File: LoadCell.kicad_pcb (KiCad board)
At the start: 2 copper layers, 51.1 x 18.5 mm, 62 parts, among them J1 M20-8760242, J2 0.100_1X4, J3 M20-8760242, J4 0.100_1X4, J5 M20-8760242, J6 0.100_1X4, J7 M20-8760242, J8 0.100_1X4, U1 L78L12ABUTR, U2 LM321SN3T1G, U3 L78L12ABUTR, U4 LM321SN3T1G, U5 L78L12ABUTR, U6 LM321SN3T1G, U7 L78L12ABUTR, U8 LM321SN3T1G

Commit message: Submitted to OSHpark
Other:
- rule pad_to_mask_clearance: 0.2 -> 0.0762
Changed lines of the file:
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@@
     (links 99)
     (no_connects 0)
-    (area 101.524999 82.982999 152.729001 101.675001)
+    (area 99.1 81.637 154.910797 105.713857)
     (thickness 1.6)
     (drawings 9)
@@
     (pad_size 1.45 1.45)
     (pad_drill 0.9)
-    (pad_to_mask_clearance 0.2)
+    (pad_to_mask_clearance 0.0762)
+    (solder_mask_min_width 0.0254)
+    (pad_to_paste_clearance -0.0254)
     (aux_axis_origin 101.6 101.6)
     (visible_elements FFFFFF7F)
     (pcbplotparams
-      (layerselection 0x00030_80000001)
+      (layerselection 0x010fc_80000001)
       (usegerberextensions false)
       (excludeedgelayer true)
@@
       (psnegative false)
       (psa4output false)
-      (plotreference true)
+      (plotreference false)
       (plotvalue true)
       (plotinvisibletext false)
@@
       (outputformat 1)
       (mirror false)
-      (drillshape 1)
+      (drillshape 0)
       (scaleselection 1)
-      (outputdirectory ""))
+      (outputdirectory ProjectOutputs/))
   )
   (net 0 "")

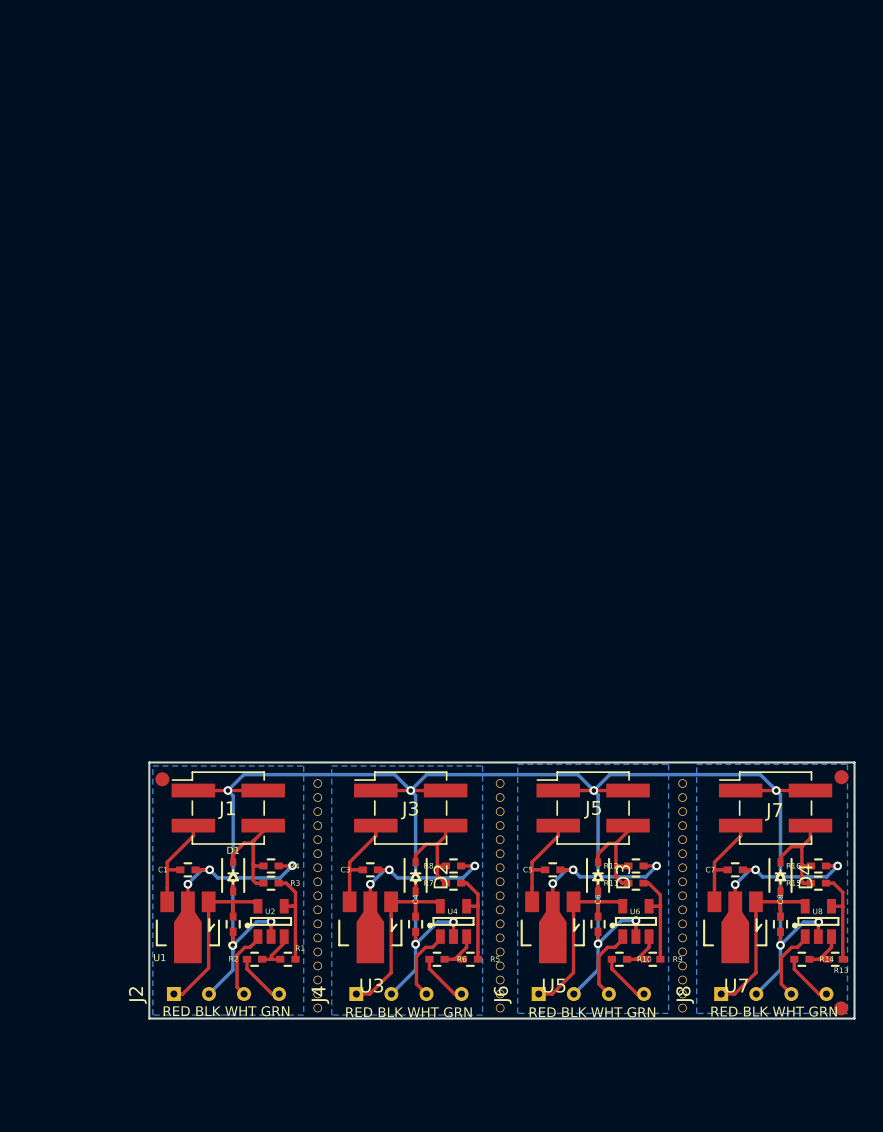
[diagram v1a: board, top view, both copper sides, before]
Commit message: Checkpoint
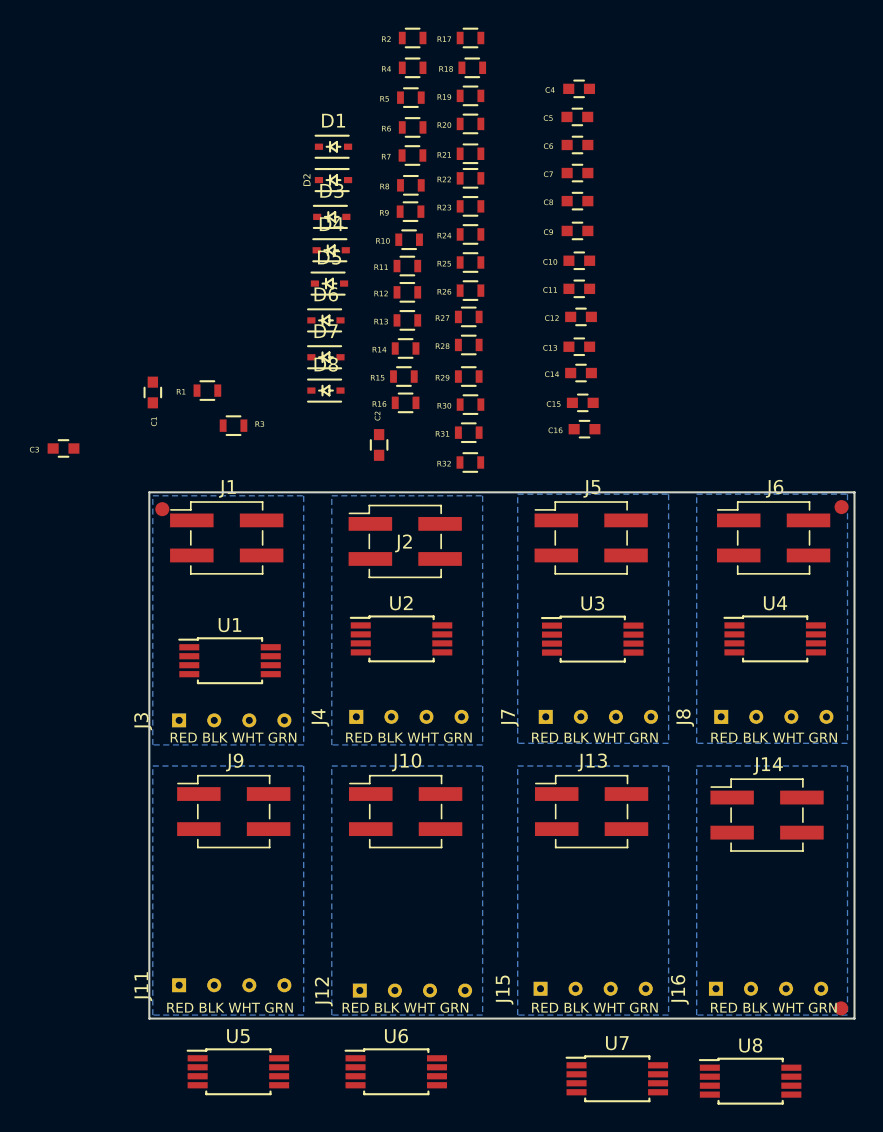
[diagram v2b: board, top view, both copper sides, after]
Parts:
- removed the D2 at (120.9, 91.3)
- removed the J4 at (120.4, 99.8)
- removed REF** (x9): Mousebites_0.020, _Connector:Mousebites__0.020
- removed mb** (x6): Mousebite_0.020, _Connector:Mousebite__0.020
- added C10: 1uF, _Passive:C_0603, F.Cu at (132.7, 46.7)
- added C11: 1uF, _Passive:C_0603, F.Cu at (132.7, 48.8)
- added C12: 1uF, _Passive:C_0603, F.Cu at (132.9, 50.8)
- added C13: 1uF, _Passive:C_0603, F.Cu at (132.7, 53.0)
- added C14: 1uF, _Passive:C_0603, F.Cu at (132.9, 54.9)
- added C15: 1uF, _Passive:C_0603, F.Cu at (133.0, 57.0)
- added C16: 1uF, _Passive:C_0603, F.Cu at (133.1, 58.9)
- added C9: 1uF, _Passive:C_0603, F.Cu at (132.6, 44.6)
- added D1: MM3Z3V0ST1G, _Passive:SOD-323, F.Cu at (114.9, 38.5)
- added D5: MM3Z3V0ST1G, _Passive:SOD-323, F.Cu at (114.6, 48.4)
- added D6: MM3Z3V0ST1G, _Passive:SOD-323, F.Cu at (114.4, 51.1)
- added D7: MM3Z3V0ST1G, _Passive:SOD-323, F.Cu at (114.4, 53.7)
- added D8: MM3Z3V0ST1G, _Passive:SOD-323, F.Cu at (114.4, 56.1)
- added J1: M20-8760242, _Connector:Pin_Header_Straight_2x02_Pitch2.54mm_SMD, F.Cu at (107.2, 66.8)
- added J10: M20-8760242, _Connector:Pin_Header_Straight_2x02_Pitch2.54mm_SMD, F.Cu at (120.2, 86.6)
- added J11: 0.100_1X4, _Connector:0.100_1x4_micro, F.Cu at (107.6, 99.2)
- added J12: 0.100_1X4, _Connector:0.100_1x4_micro, F.Cu at (120.7, 99.6)
- added J13: M20-8760242, _Connector:Pin_Header_Straight_2x02_Pitch2.54mm_SMD, F.Cu at (133.6, 86.6)
- added J14: M20-8760242, _Connector:Pin_Header_Straight_2x02_Pitch2.54mm_SMD, F.Cu at (146.3, 86.9)
- added J15: 0.100_1X4, _Connector:0.100_1x4_micro, F.Cu at (133.7, 99.4)
- added J16: 0.100_1X4, _Connector:0.100_1x4_micro, F.Cu at (146.4, 99.4)
- added J9: M20-8760242, _Connector:Pin_Header_Straight_2x02_Pitch2.54mm_SMD, F.Cu at (107.7, 86.6)
- added R17: 390K, _Passive:R_0603, F.Cu at (124.9, 30.6)
- added R18: 1K, _Passive:R_0603, F.Cu at (125.0, 32.8)
- added R19: 390K, _Passive:R_0603, F.Cu at (124.9, 34.8)
- added R20: 1K, _Passive:R_0603, F.Cu at (124.9, 36.8)
- added R21: 1K, _Passive:R_0603, F.Cu at (124.9, 39.0)
- added R22: 270K, _Passive:R_0603, F.Cu at (124.9, 40.8)
- added R23: 1K, _Passive:R_0603, F.Cu at (124.9, 42.8)
- added R24: 270K, _Passive:R_0603, F.Cu at (124.9, 44.8)
- added R25: 390K, _Passive:R_0603, F.Cu at (124.9, 46.9)
- added R26: 1K, _Passive:R_0603, F.Cu at (124.9, 48.9)
- added R27: 390K, _Passive:R_0603, F.Cu at (124.7, 50.8)
- added R28: 1K, _Passive:R_0603, F.Cu at (124.7, 52.8)
- added R29: 1K, _Passive:R_0603, F.Cu at (124.7, 55.1)
- added R30: 270K, _Passive:R_0603, F.Cu at (124.9, 57.1)
- added R31: 1K, _Passive:R_0603, F.Cu at (124.7, 59.2)
- added R32: 270K, _Passive:R_0603, F.Cu at (124.8, 61.3)
- C1, C2, C3, C4, C5, C6, C7, C8: footprint _Passive:C_0402 -> _Passive:C_0603
- J3, J7: value M20-8760242 -> 0.100_1X4; footprint _Connector:Pin_Header_Straight_2x02_Pitch2.54mm_SMD -> _Connector:0.100_1x4_micro
- J6: value 0.100_1X4 -> M20-8760242; footprint _Connector:0.100_1x4_micro -> _Connector:Pin_Header_Straight_2x02_Pitch2.54mm_SMD
- R1, R9: value 270K -> 390K; footprint _Passive:R_0402 -> _Passive:R_0603
- R10, R2: footprint _Passive:R_0402 -> _Passive:R_0603
- R11, R3: value 100R -> 390K; footprint _Passive:R_0402 -> _Passive:R_0603
- R12, R15, R4, R7: value 100R -> 1K; footprint _Passive:R_0402 -> _Passive:R_0603
- R13, R5: value 270K -> 1K; footprint _Passive:R_0402 -> _Passive:R_0603
- R14, R6: value 1K -> 270K; footprint _Passive:R_0402 -> _Passive:R_0603
- R16, R8: value 100R -> 270K; footprint _Passive:R_0402 -> _Passive:R_0603
- U1, U3, U5, U7: value L78L12ABUTR -> MCP6002; footprint _Active:SOT89-3 -> Housings_SSOP:TSSOP-8_4.4x3mm_Pitch0.65mm
- U2, U4, U6, U8: value LM321SN3T1G -> MCP6002; footprint _Active:SOT-23-5 -> Housings_SSOP:TSSOP-8_4.4x3mm_Pitch0.65mm
- moved R2 67.7 mm to (120.7, 30.6), turned to 0 degrees
- moved R5 62.5 mm to (120.5, 34.9), turned to 0 degrees
- moved C4 61.6 mm to (132.7, 34.3), turned to 0 degrees
- moved R6 60.2 mm to (120.7, 37.1), turned to 0 degrees
- moved R4 58.7 mm to (120.7, 32.8)
- moved R9 56.9 mm to (120.5, 43.2), turned to 0 degrees
- moved C6 56.4 mm to (132.6, 38.4), turned to 0 degrees
- moved D4 55.8 mm to (114.8, 46.0), turned to 0 degrees
- moved R13 55.7 mm to (120.3, 51.1), turned to 0 degrees
- moved C5 54.5 mm to (132.6, 36.3)
- moved C8 54.4 mm to (132.6, 42.4), turned to 0 degrees
- moved R10 54.3 mm to (120.4, 45.2), turned to 0 degrees
- moved R7 52.8 mm to (120.7, 39.1)
- moved R14 52.7 mm to (120.2, 53.1), turned to 0 degrees
- moved C7 51.7 mm to (132.6, 40.4)
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- renumbered D1 to D2, J1 to J2, J2 to J4
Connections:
- C1 pad 1: /Main Sheet/Vin -> /Main Sheet/Vout
- C1 pad 2: GND -> /Main Sheet/BLK
- C2 pad 1: /Main Sheet/RED -> /Main Sheet/Vout
- C2 pad 2: GND -> /Main Sheet/BLK
- C3 pad 1: Net-(C3-Pad1) -> /Main Sheet/RED
- C3 pad 2: GND -> /Main Sheet/BLK
- C4 pad 1: Net-(C4-Pad1) -> /Main Sheet/RED
- C4 pad 2: GND -> /Main Sheet/BLK
- C5 pad 1: Net-(C5-Pad1) -> /Main Sheet/Vout
- C5 pad 2: GND -> /Main Sheet/BLK
- C6 pad 1: Net-(C6-Pad1) -> /Main Sheet/Vout
- C6 pad 2: GND -> /Main Sheet/BLK
- C7 pad 1: Net-(C7-Pad1) -> /Main Sheet/RED
- C7 pad 2: GND -> /Main Sheet/BLK
- C8 pad 1: Net-(C8-Pad1) -> /Main Sheet/RED
- C8 pad 2: GND -> /Main Sheet/BLK
- D2 pad 2: GND -> /Main Sheet/BLK
- D3 pad 1: Net-(D3-Pad1) -> /Main Sheet/Vout
- D3 pad 2: GND -> /Main Sheet/BLK
- D4 pad 1: Net-(D4-Pad1) -> /Main Sheet/Vout
- D4 pad 2: GND -> /Main Sheet/BLK
- FID1 pad 1: Net-(FID1-Pad1) -> (no net)
- FID2 pad 1: Net-(FID2-Pad1) -> (no net)
- FID3 pad 1: Net-(FID3-Pad1) -> (no net)
- J2 pad 1: GND -> /Main Sheet/BLK
- J2 pad 2: GND -> /Main Sheet/BLK
- J2 pad 3: /Main Sheet/Vin -> /Main Sheet/RED
- J3 pad 1: GND -> /Main Sheet/RED
- J3 pad 2: GND -> /Main Sheet/BLK
- J3 pad 3: Net-(C3-Pad1) -> /Main Sheet/WHT
- J3 pad 4: Net-(D2-Pad1) -> /Main Sheet/GRN
- J4 pad 2: GND -> /Main Sheet/BLK
- J4 pad 3: /Main Sheet/VL+ -> /Main Sheet/WHT
- J5 pad 1: GND -> /Main Sheet/BLK
- J5 pad 2: GND -> /Main Sheet/BLK
- J5 pad 3: Net-(C5-Pad1) -> /Main Sheet/RED
- J5 pad 4: Net-(D3-Pad1) -> /Main Sheet/Vout
- J6 pad 1: Net-(C6-Pad1) -> /Main Sheet/BLK
- J6 pad 2: GND -> /Main Sheet/BLK
- J6 pad 3: Net-(J6-Pad3) -> /Main Sheet/RED
- J6 pad 4: Net-(J6-Pad4) -> /Main Sheet/Vout
- J7 pad 1: GND -> /Main Sheet/RED
- J7 pad 2: GND -> /Main Sheet/BLK
- J7 pad 3: Net-(C7-Pad1) -> /Main Sheet/WHT
- J7 pad 4: Net-(D4-Pad1) -> /Main Sheet/GRN
- J8 pad 1: Net-(C8-Pad1) -> /Main Sheet/RED
- J8 pad 2: GND -> /Main Sheet/BLK
- J8 pad 3: Net-(J8-Pad3) -> /Main Sheet/WHT
- J8 pad 4: Net-(J8-Pad4) -> /Main Sheet/GRN
- R1 pad 1: /Main Sheet/Vopo -> Net-(R1-Pad1)
- R1 pad 2: /Main Sheet/VL- -> Net-(R1-Pad2)
- R10 pad 2: Net-(J6-Pad4) -> /Main Sheet/Vout
- R11 pad 1: Net-(D3-Pad1) -> Net-(R11-Pad1)
- R12 pad 1: Net-(D3-Pad1) -> Net-(R12-Pad1)
- R12 pad 2: GND -> /Main Sheet/Vout
- R13 pad 1: Net-(R13-Pad1) -> /Main Sheet/Vout
- R14 pad 1: Net-(R13-Pad2) -> /Main Sheet/BLK
- R14 pad 2: Net-(J8-Pad4) -> Net-(R10-Pad1)
- R15 pad 1: Net-(D4-Pad1) -> /Main Sheet/Vout
- R15 pad 2: Net-(R13-Pad1) -> Net-(R11-Pad1)
- R16 pad 1: Net-(D4-Pad1) -> /Main Sheet/BLK
- R16 pad 2: GND -> Net-(R12-Pad1)
- R2 pad 1: /Main Sheet/VL- -> Net-(R2-Pad1)
- R2 pad 2: /Main Sheet/GRN -> /Main Sheet/Vout
- R3 pad 1: /Main Sheet/Vout -> Net-(R3-Pad1)
- R3 pad 2: /Main Sheet/Vopo -> Net-(R3-Pad2)
- R4 pad 1: /Main Sheet/Vout -> Net-(R4-Pad1)
- R4 pad 2: GND -> /Main Sheet/Vout
- R5 pad 1: Net-(R5-Pad1) -> /Main Sheet/Vout
- R5 pad 2: Net-(R5-Pad2) -> Net-(R1-Pad1)
- R6 pad 1: Net-(R5-Pad2) -> /Main Sheet/BLK
- R6 pad 2: Net-(J4-Pad4) -> Net-(R2-Pad1)
- R7 pad 1: Net-(D2-Pad1) -> /Main Sheet/Vout
- R7 pad 2: Net-(R5-Pad1) -> Net-(R3-Pad1)
- R8 pad 1: Net-(D2-Pad1) -> /Main Sheet/BLK
- R8 pad 2: GND -> Net-(R4-Pad1)
- R9 pad 1: Net-(R11-Pad2) -> Net-(R13-Pad2)
- R9 pad 2: Net-(R10-Pad1) -> Net-(R9-Pad2)
- U1 pad 1: /Main Sheet/RED -> Net-(R1-Pad2)
- U1 pad 2: GND -> Net-(R1-Pad1)
- U1 pad 3: /Main Sheet/Vin -> /Main Sheet/GRN
- U2 pad 1: /Main Sheet/VL+ -> Net-(R3-Pad2)
- U2 pad 2: GND -> Net-(R3-Pad1)
- U2 pad 3: /Main Sheet/VL- -> /Main Sheet/GRN
- U2 pad 4: /Main Sheet/Vopo -> /Main Sheet/BLK
- U2 pad 5: /Main Sheet/RED -> /Main Sheet/WHT
- U3 pad 1: Net-(C4-Pad1) -> Net-(R9-Pad2)
- U3 pad 2: GND -> Net-(R13-Pad2)
- U3 pad 3: Net-(C3-Pad1) -> /Main Sheet/GRN
- U4 pad 1: Net-(J4-Pad3) -> Net-(R11-Pad2)
- U4 pad 2: GND -> Net-(R11-Pad1)
- U4 pad 3: Net-(R5-Pad2) -> /Main Sheet/GRN
- U4 pad 4: Net-(R5-Pad1) -> /Main Sheet/BLK
- U4 pad 5: Net-(C4-Pad1) -> /Main Sheet/WHT
- U5 pad 1: Net-(C6-Pad1) -> Net-(R17-Pad2)
- U5 pad 2: GND -> Net-(R17-Pad1)
- U5 pad 3: Net-(C5-Pad1) -> /Main Sheet/GRN
- U6 pad 1: Net-(J6-Pad3) -> Net-(R19-Pad2)
- U6 pad 2: GND -> Net-(R19-Pad1)
- U6 pad 3: Net-(R10-Pad1) -> /Main Sheet/GRN
- U6 pad 4: Net-(R11-Pad2) -> /Main Sheet/BLK
- U6 pad 5: Net-(C6-Pad1) -> /Main Sheet/WHT
- U7 pad 1: Net-(C8-Pad1) -> Net-(R25-Pad2)
- U7 pad 2: GND -> Net-(R25-Pad1)
- U7 pad 3: Net-(C7-Pad1) -> /Main Sheet/GRN
- U8 pad 1: Net-(J8-Pad3) -> Net-(R27-Pad2)
- U8 pad 2: GND -> Net-(R27-Pad1)
- U8 pad 3: Net-(R13-Pad2) -> /Main Sheet/GRN
- U8 pad 4: Net-(R13-Pad1) -> /Main Sheet/BLK
- U8 pad 5: Net-(C8-Pad1) -> /Main Sheet/WHT
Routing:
- net GND: track 210.7 -> 0.00 mm, vias 28 -> 0
- net Net-(C8-Pad1): track 13.1 -> 0.00 mm
- net Net-(C6-Pad1): track 13.1 -> 0.00 mm
- net Net-(C4-Pad1): track 13.1 -> 0.00 mm
- net /Main Sheet/RED: track 12.9 -> 0.00 mm
- net /Main Sheet/Vout: track 8.46 -> 0.00 mm
- net Net-(D3-Pad1): track 8.27 -> 0.00 mm
- net Net-(D4-Pad1): track 7.93 -> 0.00 mm
- net Net-(D2-Pad1): track 7.75 -> 0.00 mm
- net Net-(C3-Pad1): track 7.26 -> 0.00 mm
- net Net-(C7-Pad1): track 7.26 -> 0.00 mm
- net /Main Sheet/Vin: track 7.25 -> 0.00 mm
- net Net-(C5-Pad1): track 7.25 -> 0.00 mm
- net Net-(R5-Pad1): track 7.18 -> 0.00 mm
- net Net-(R13-Pad1): track 7.17 -> 0.00 mm
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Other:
- board size 51.1 x 18.5 mm -> 51.1 x 38.1 mm
